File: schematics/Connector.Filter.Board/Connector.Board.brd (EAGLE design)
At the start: 160 x 100 mm, 72 parts

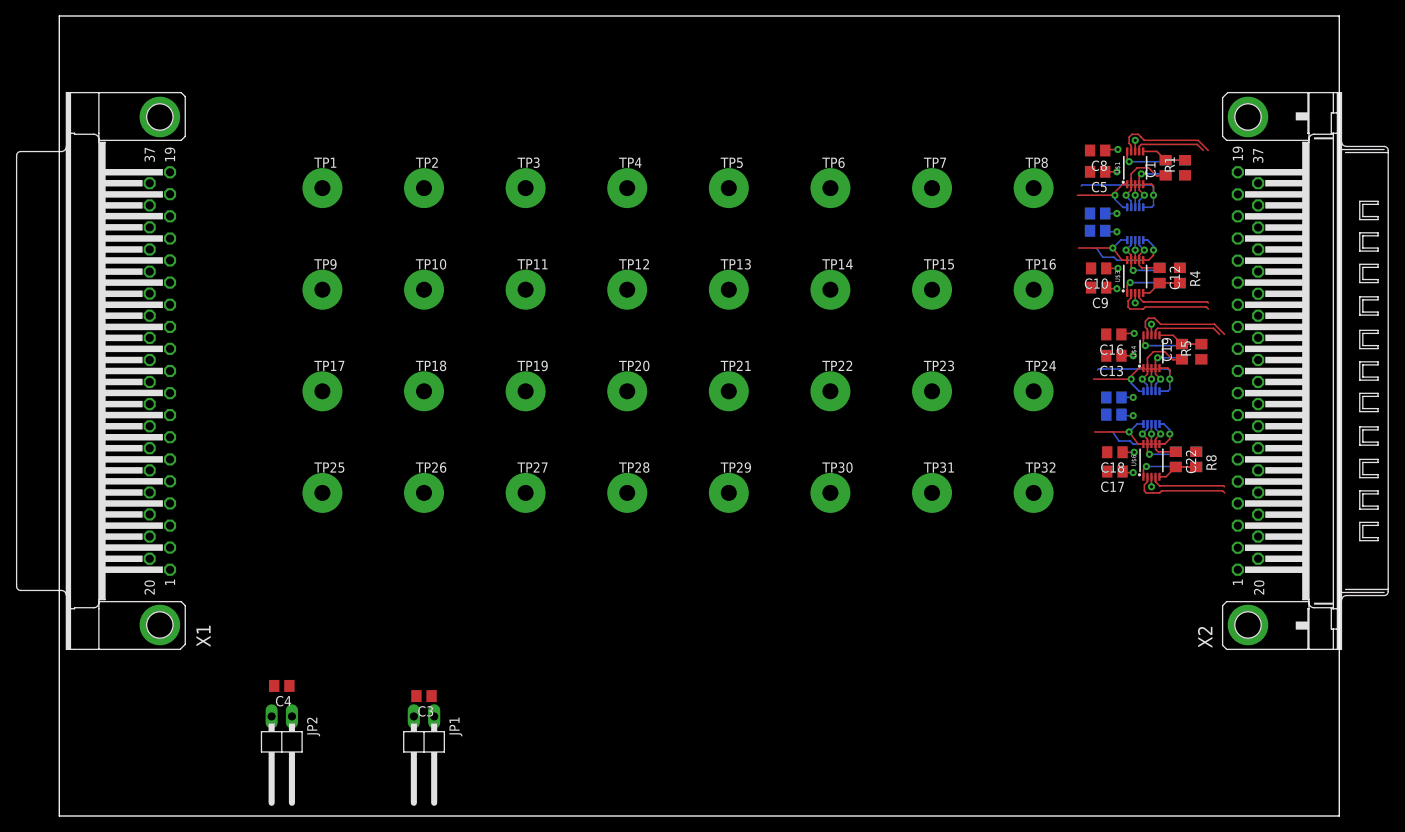
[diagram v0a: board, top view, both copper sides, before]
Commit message: 12 chn board finished
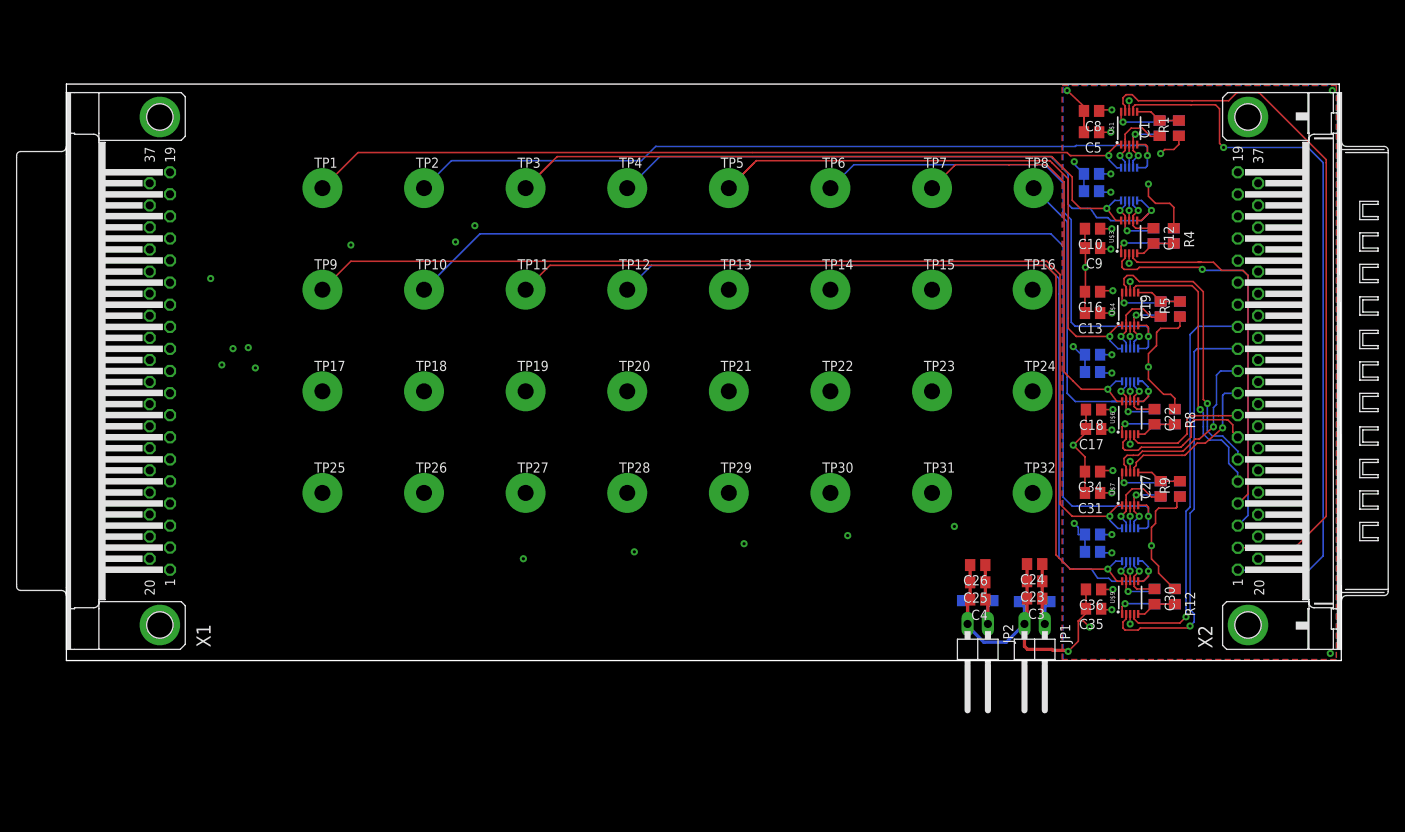
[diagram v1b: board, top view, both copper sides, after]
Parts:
- added C23, C24, C25, C26, C27, C28, C29, C30, C31, C32, C33, C34, C35, C36: (no value), resistor:C0805
- added D1, D3: 1N4148W-7-F, diode:SOD123
- added R10, R11, R12, R9: (no value), resistor:R0805
- added U$7, U$8, U$9: AD8244, AD8244:MSOP10
- moved JP2 87.8 mm to (114.8, 20.2)
- moved C4 87.7 mm to (114.8, 27.1)
- moved C3 77.3 mm to (121.9, 27.2)
- moved JP1 77.2 mm to (121.9, 20.2)
- moved C13 5.96 mm to (129.2, 62.9)
- moved C14 5.96 mm to (129.2, 57.7)
- moved C15 5.96 mm to (129.2, 55.5)
- moved C17 5.96 mm to (129.3, 48.4)
- moved C21 5.96 mm to (136.9, 49.9)
- moved C22 5.96 mm to (136.9, 49.9)
- moved R7 5.96 mm to (139.4, 49.9)
- moved R8 5.96 mm to (139.4, 49.9)
- moved C16 5.96 mm to (129.2, 65.5)
- moved C18 5.96 mm to (129.3, 50.8)
- moved C19 5.96 mm to (137.7, 63.4)
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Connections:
- removed net VDD: C10.1, C15.1, C16.1, C18.1, C4.1, C7.1, C8.1, JP2.1, U$1.8, U$2.8, U$3.8, U$4.8, U$5.8, U$6.8
- removed net VSS: C13.1, C14.1, C17.1, C3.1, C5.1, C6.1, C9.1, JP1.1, U$1.3, U$2.3, U$3.3, U$4.3, U$5.3, U$6.3
- new net BUF10: C28.1, U$7.4, U$8.4
- new net BUF11: C29.1, U$8.9, U$9.9
- new net BUF12: C30.1, U$8.7, U$9.7
- new net BUF9: C27.1, U$7.2, U$8.2
- new net FILT10_OUT: C28.2, R10.2, U$7.10
- new net FILT11_OUT: C29.2, R11.2, U$9.1
- new net FILT12_OUT: C30.2, R12.2, U$9.5
- new net FILT9_OUT: C27.2, R9.2, U$7.6
- new net V+: C13.1, C14.1, C17.1, C23.1, C24.1, C3.1, C31.1, C32.1, C35.1, C5.1, C6.1, C9.1, D1.C, JP1.1, U$1.3, U$2.3, U$3.3, U$4.3, U$5.3, U$6.3, U$7.3, U$8.3, U$9.3
- new net V-: C10.1, C15.1, C16.1, C18.1, C25.1, C26.1, C33.1, C34.1, C36.1, C4.1, C7.1, C8.1, D3.A, JP2.1, U$1.8, U$2.8, U$3.8, U$4.8, U$5.8, U$6.8, U$7.8, U$8.8, U$9.8
- net FILT10_BUF: now also U$7.9
- net FILT11_BUF: now also U$9.2
- net FILT12_BUF: now also U$9.4
- net FILT9_BUF: now also U$7.7
- net GND: now also C23.2, C24.2, C25.2, C26.2, C31.2, C32.2, C33.2, C34.2, C35.2, C36.2, D1.A, D3.C, R10.1, R11.1, R12.1, R9.1
- net PIN10: now also U$7.5, U$8.5
- net PIN11: now also U$8.10, U$9.10
- net PIN12: now also U$8.6, U$9.6
- net PIN9: now also U$7.1, U$8.1
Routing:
- net GND: track 0.00 -> 310.2 mm, vias 0 -> 14
- net PIN5: track 9.76 -> 188.4 mm
- net V-: track 0.00 -> 178.3 mm, vias 0 -> 15
- net PIN7: track 9.07 -> 185.4 mm
- net PIN8: track 12.4 -> 186.9 mm
- net PIN10: track 0.00 -> 170.9 mm, vias 0 -> 2
- net PIN6: track 15.4 -> 186.0 mm
- net PIN12: track 0.00 -> 170.3 mm, vias 0 -> 2
- net PIN9: track 0.00 -> 169.9 mm, vias 0 -> 2
- net PIN3: track 9.07 -> 177.5 mm
- net PIN4: track 12.4 -> 180.4 mm
- net V+: track 0.00 -> 165.1 mm, vias 0 -> 15
- net PIN11: track 0.00 -> 164.1 mm, vias 0 -> 2
- net PIN2: track 15.4 -> 179.1 mm
- net PIN1: track 9.76 -> 167.9 mm
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- added copper zone on layer 1, net GND
- added copper zone on layer 16, net GND
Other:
- board size 160 x 100 mm -> 159.4 x 72.1 mm
